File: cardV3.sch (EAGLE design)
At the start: 66 parts, among them IC1 ATTINY1616, IC2 LTC1992-1, IC3 LTC1992, IC4 LTC6911, IC5 LTC2402, SW1 SPST_TACT-EVQQ2, SW2 SPST_TACT-EVQQ2, SW3 SPST_TACT-EVQQ2, SW4 SPST_TACT-EVQQ2

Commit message: Better V3...
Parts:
- removed C2.1, C3.1: 1u, resistor:C-USC0805
- removed C4.1: 1u, adafruit:CPOL-USA/3216-18R
- removed GA, GB: TPSQB1,27, testpad:TPSQB1,27
- removed IC5: LTC2402, HomeMade:LTC2402CMS
- removed PIN: (no value), con-amp:MTA03-100
- removed R21, R22, R31, R32: 470k, resistor:R-US_M0805
- removed R23, R33: 10k, resistor:R-US_M0805
- removed R24, R34: 1, resistor:R-US_M0805
- removed R29, R39: 100, resistor:R-US_M0805
- removed RESA, RESB: (no value), con-phoenix-254:MPT2
- removed SJ1, SJ2: (no value), jumper:SJ
- removed U$1: NOKIA_SCREEN, HomeMade:NOKIA_SCREEN
- added GAN, VAN: (no value), jumper:SJ
- added PA7: TPSQB1,27, testpad:TPSQB1,27
- added R1A, R1B, R2A, R2B: 1M, resistor:R-US_M0805
- added R3A, R3B, R4A, R4B: 390k, resistor:R-US_M0805
- added R5A, R5B, R6A, R6B: 100k, resistor:R-US_M0805
- added RA, RB: 1, resistor:R-US_M0805
- added SCR: NOKIA_SCREEN, HomeMade:NOKIA_SCREEN
- IC2: value LTC1992-1 -> AD8231; device linear-technology-2:LTC1992CMS8 -> HomeMade:AD8231
- IC3: value LTC1992 -> AD8231; device linear-technology-2:LTC1992CMS8 -> HomeMade:AD8231
- IC4: value LTC6911 -> LTC2402; device HomeMade:LTC6911CMS-1 -> HomeMade:LTC2402CMS
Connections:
- removed net G0: IC1.PA4, IC4.G0
- removed net G1: IC1.PA5, IC4.G1
- removed net G2: IC1.PA6, IC4.G2
- removed net N$21: C2.1.1, IC2G$1.MID, IC2G$1.OCM
- removed net N$22: R21.2, R22.1
- removed net N$25: AMPB-1.1, IC3G$1.-IN, R33.2, R34.1, VB-.TP
- removed net N$26: IC3G$1.+IN, R32.2, R33.1, RESB-1.1, VB+.TP
- removed net N$27: R21.1, VOLTA-1.1
- removed net N$28: R29.1, RESA-2.1
- removed net N$29: GB.TP, IC4.OUTB, IC5.CH0
- removed net N$31: C3.1.1, IC3G$1.MID, IC3G$1.OCM
- removed net N$32: R31.2, R32.1
- removed net N$35: R31.1, VOLTB-1.1
- removed net N$36: R39.1, RESB-2.1
- removed net N$37: GA.TP, IC4.OUTA, IC5.CH1
- removed net RAWA: IC2G$1.-OUT, IC4.INA, VA.TP
- removed net RAWB: IC3G$1.-OUT, IC4.INB, VB.TP
- new net A0: IC1.PA4, IC2.A0, IC3.A0
- new net A1: IC1.PA5, IC2.A1, IC3.A1
- new net A2: IC1.PA6, IC2.A2, IC3.A2
- new net N$10: IC2.+INB, R5A.1, R6A.2
- new net N$11: R3A.1, VOLTA-2.1
- new net N$12: AMPA-2.1, IC2.-INA, R1A.2, R3A.2, RA.1, VA-.TP
- new net N$13: IC2.-INB, IC2.OUTB, IC2.REF
- new net N$14: AMPA-1.1, IC2.+INA, R2A.1, R4A.2, RA.2, VA+.TP
- new net N$15: R3B.1, VOLTB-2.1
- new net N$19: IC1.PA7, PA7.TP
- new net VA: IC2.OUTA, IC4.CH1, VA.TP
- new net VB: IC3.OUTA, IC4.CH0, VB.TP
- new net _CS_INA: IC1.PB5, IC2._CS
- new net _CS_INB: IC1.PB4, IC3._CS
- net +3V3: now also IC4.FO, IC4.VCC, SCR.VCC1, SCR.VCC2, VAN.1; no longer IC5.FO, IC5.VCC, SJ2.1, U$1.VCC1, U$1.VCC2
- net AGND: now also GAN.2, IC2.-VS, IC2.PAD, IC3.-VS, IC3.PAD, IC4.ZSET, R1A.1, R1B.1, R2A.2, R2B.2, R5A.2, R5B.2; no longer AMPA-2.1, AMPB-2.1, C2.1.2, C3.1.2, C4.1.-, IC2P.VEE, IC3P.VEE, IC4.V-, IC5.ZSET, R24.2, R34.2, SJ1.2, VOLTA-2.1, VOLTB-2.1
- net CLK: now also IC4.SCK, SCR.CLK; no longer IC5.SCK, U$1.CLK
- net D/C: now also SCR.DC; no longer U$1.DC
- net GND: now also GAN.1, IC4.GND, SCR.GND; no longer IC5.GND, SJ1.1, U$1.GND
- net MISO: now also IC4.SDO; no longer IC5.SDO
- net MOSI: now also SCR.DIN; no longer U$1.DIN
- net N$16: now also IC3.-INB, IC3.OUTB, IC3.REF; no longer AMPA-1.1, IC2G$1.-IN, R23.2, R24.1, VA-.TP
- net N$17: now also R4B.1, VOLTB-1.1; no longer IC2G$1.+IN, R22.2, R23.1, RESA-1.1, VA+.TP
- net N$18: now also IC3.+INB, R5B.1, R6B.2; no longer C4.1.+, IC4.AGND
- net N$3: now also SCR.CAP; no longer U$1.CAP
- net N$7: now also R4A.1, VOLTA-1.1; no longer IC1.PB4, PIN.1
- net N$8: now also AMPB-2.1, IC3.-INA, R1B.2, R3B.2, RB.1, VB-.TP; no longer IC1.PA7, PIN.3
- net N$9: now also AMPB-1.1, IC3.+INA, R2B.1, R4B.2, RB.2, VB+.TP; no longer IC1.PB5, PIN.2
- net RST: now also SCR.RST; no longer U$1.RST
- net V+: now also IC2.+VS, IC2._SDN, IC3.+VS, IC3._SDN, IC4.FSET, R6A.1, R6B.1, VAN.2; no longer IC2P.VDD, IC3P.VDD, IC4.V+, IC5.FSET, R29.2, R39.2, SJ2.2
- net _CS_ADC: now also IC4.~CS; no longer IC5.~CS
- net _CS_SCR: now also SCR.CE; no longer U$1.CE
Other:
- note removed: "Input impedance of 1-10k"
- moved on the sheet: AMPA-1, AMPA-2, AMPB-1, AMPB-2, C1, C2, C3, C4, C5, C6, CLK, CS_A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

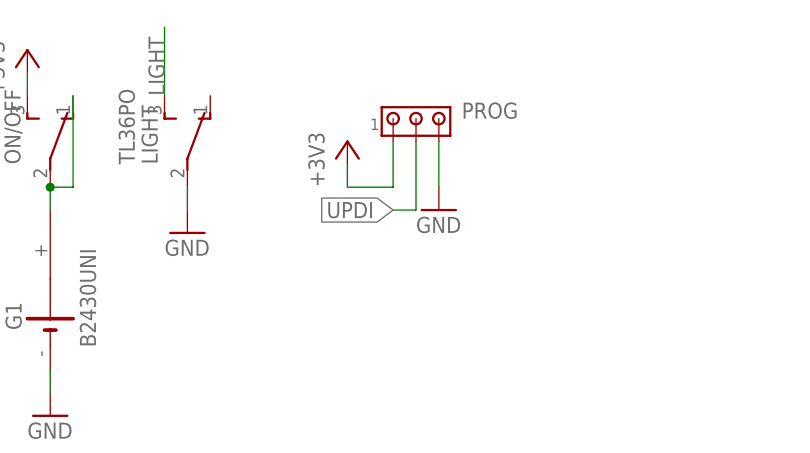
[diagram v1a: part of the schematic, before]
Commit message: improvement
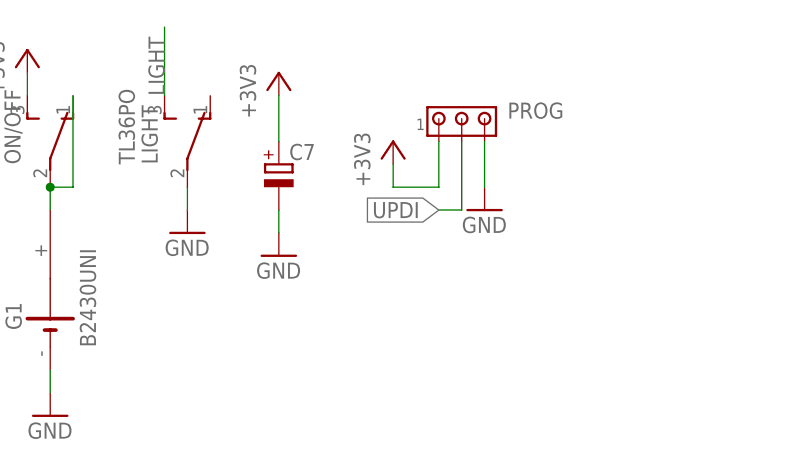
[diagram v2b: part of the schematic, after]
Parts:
- added C7: (no value), rcl:CPOL-EU153CLV-0405
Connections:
- net +3V3: now also C7.+
- net GND: now also C7.-
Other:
- moved on the sheet: PROG
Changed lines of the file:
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@@
 <setting verticaltext="up"/>
 </settings>
-<grid distance="0.1" unitdist="inch" unit="inch" style="lines" multiple="1" display="yes" altdistance="0.01" altunitdist="inch" altunit="inch"/>
+<grid distance="0.1" unitdist="inch" unit="inch" style="lines" multiple="1" display="no" altdistance="0.01" altunitdist="inch" altunit="inch"/>
 <layers>
 <layer number="1" name="Top" color="4" fill="1" visible="no" active="no"/>
@@
 <part name="AGND14" library="supply1" deviceset="AGND" device=""/>
 <part name="AGND15" library="supply1" deviceset="AGND" device=""/>
+<part name="C7" library="rcl" deviceset="CPOL-EU" device="153CLV-0405"/>
+<part name="+3V8" library="supply1" deviceset="+3V3" device=""/>
+<part name="GND5" library="supply1" deviceset="GND" device=""/>
 </parts>
 <sheets>
@@
 <instance part="+3V16" gate="G$1" x="137.16" y="86.36"/>
 <instance part="GND23" gate="1" x="137.16" y="73.66"/>
-<instance part="PROG" gate="G$1" x="142.24" y="198.12"/>
-<instance part="+3V17" gate="G$1" x="134.62" y="195.58"/>
-<instance part="GND24" gate="1" x="144.78" y="187.96"/>
+<instance part="PROG" gate="G$1" x="147.32" y="198.12"/>
+<instance part="+3V17" gate="G$1" x="139.7" y="195.58"/>
+<instance part="GND24" gate="1" x="149.86" y="187.96"/>
 <instance part="VA+" gate="G$1" x="50.8" y="111.76"/>
 <instance part="VA-" gate="G$1" x="50.8" y="132.08" rot="R180"/>
@@
 <instance part="AGND14" gate="VR1" x="93.98" y="109.22"/>
 <instance part="AGND15" gate="VR1" x="93.98" y="33.02"/>
+<instance part="C7" gate="G$1" x="127" y="193.04"/>
+<instance part="+3V8" gate="G$1" x="127" y="203.2"/>
+<instance part="GND5" gate="1" x="127" y="182.88"/>
 </instances>
 <busses>
@@
 <segment>
 <pinref part="PROG" gate="G$1" pin="1"/>
-<wire x1="139.7" y1="195.58" x2="139.7" y2="190.5" width="0.1524" layer="91"/>
+<wire x1="144.78" y1="195.58" x2="144.78" y2="190.5" width="0.1524" layer="91"/>
 <pinref part="+3V17" gate="G$1" pin="+3V3"/>
-<wire x1="139.7" y1="190.5" x2="134.62" y2="190.5" width="0.1524" layer="91"/>
-<wire x1="134.62" y1="190.5" x2="134.62" y2="193.04" width="0.1524" layer="91"/>
+<wire x1="144.78" y1="190.5" x2="139.7" y2="190.5" width="0.1524" layer="91"/>
+<wire x1="139.7" y1="190.5" x2="139.7" y2="193.04" width="0.1524" layer="91"/>
 </segment>
 <segment>
@@
 <pinref part="IC4" gate="G$1" pin="FO"/>
 <wire x1="157.48" y1="129.54" x2="160.02" y2="129.54" width="0.1524" layer="91"/>
+</segment>
+<segment>
+<pinref part="C7" gate="G$1" pin="+"/>
+<pinref part="+3V8" gate="G$1" pin="+3V3"/>
+<wire x1="127" y1="200.66" x2="127" y2="195.58" width="0.1524" layer="91"/>
 </segment>
 </net>
@@
 <pinref part="PROG" gate="G$1" pin="3"/>
 <pinref part="GND24" gate="1" pin="GND"/>
-<wire x1="144.78" y1="195.58" x2="144.78" y2="190.5" width="0.1524" layer="91"/>
+<wire x1="149.86" y1="195.58" x2="149.86" y2="190.5" width="0.1524" layer="91"/>
 </segment>
 <segment>
@@
 <pinref part="GAN" gate="1" pin="1"/>
 <wire x1="68.58" y1="177.8" x2="68.58" y2="180.34" width="0.1524" layer="91"/>
+</segment>
+<segment>
+<pinref part="C7" gate="G$1" pin="-"/>
+<pinref part="GND5" gate="1" pin="GND"/>
+<wire x1="127" y1="185.42" x2="127" y2="187.96" width="0.1524" layer="91"/>
 </segment>
 </net>
@@
 <segment>
 <pinref part="PROG" gate="G$1" pin="2"/>
-<wire x1="142.24" y1="195.58" x2="142.24" y2="187.96" width="0.1524" layer="91"/>
-<wire x1="142.24" y1="187.96" x2="139.7" y2="187.96" width="0.1524" layer="91"/>
-<label x="139.7" y="187.96" size="1.778" layer="95" rot="R180" xref="yes"/>
-</segment>
-</net>
+<wire x1="147.32" y1="195.58" x2="147.32" y2="187.96" width="0.1524" layer="91"/>
+<wire x1="147.32" y1="187.96" x2="144.78" y2="187.96" width="0.1524" layer="91"/>
+<label x="144.78" y="187.96" size="1.778" layer="95" rot="R180" xref="yes"/>
+</segment>
+</net>
